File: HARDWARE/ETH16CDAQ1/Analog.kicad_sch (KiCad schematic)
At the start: 15 parts, among them J401 5499141-4, U401 ADG5408BRUZ, U402 ADG5408BRUZ, U403 ADA4254ARUZ

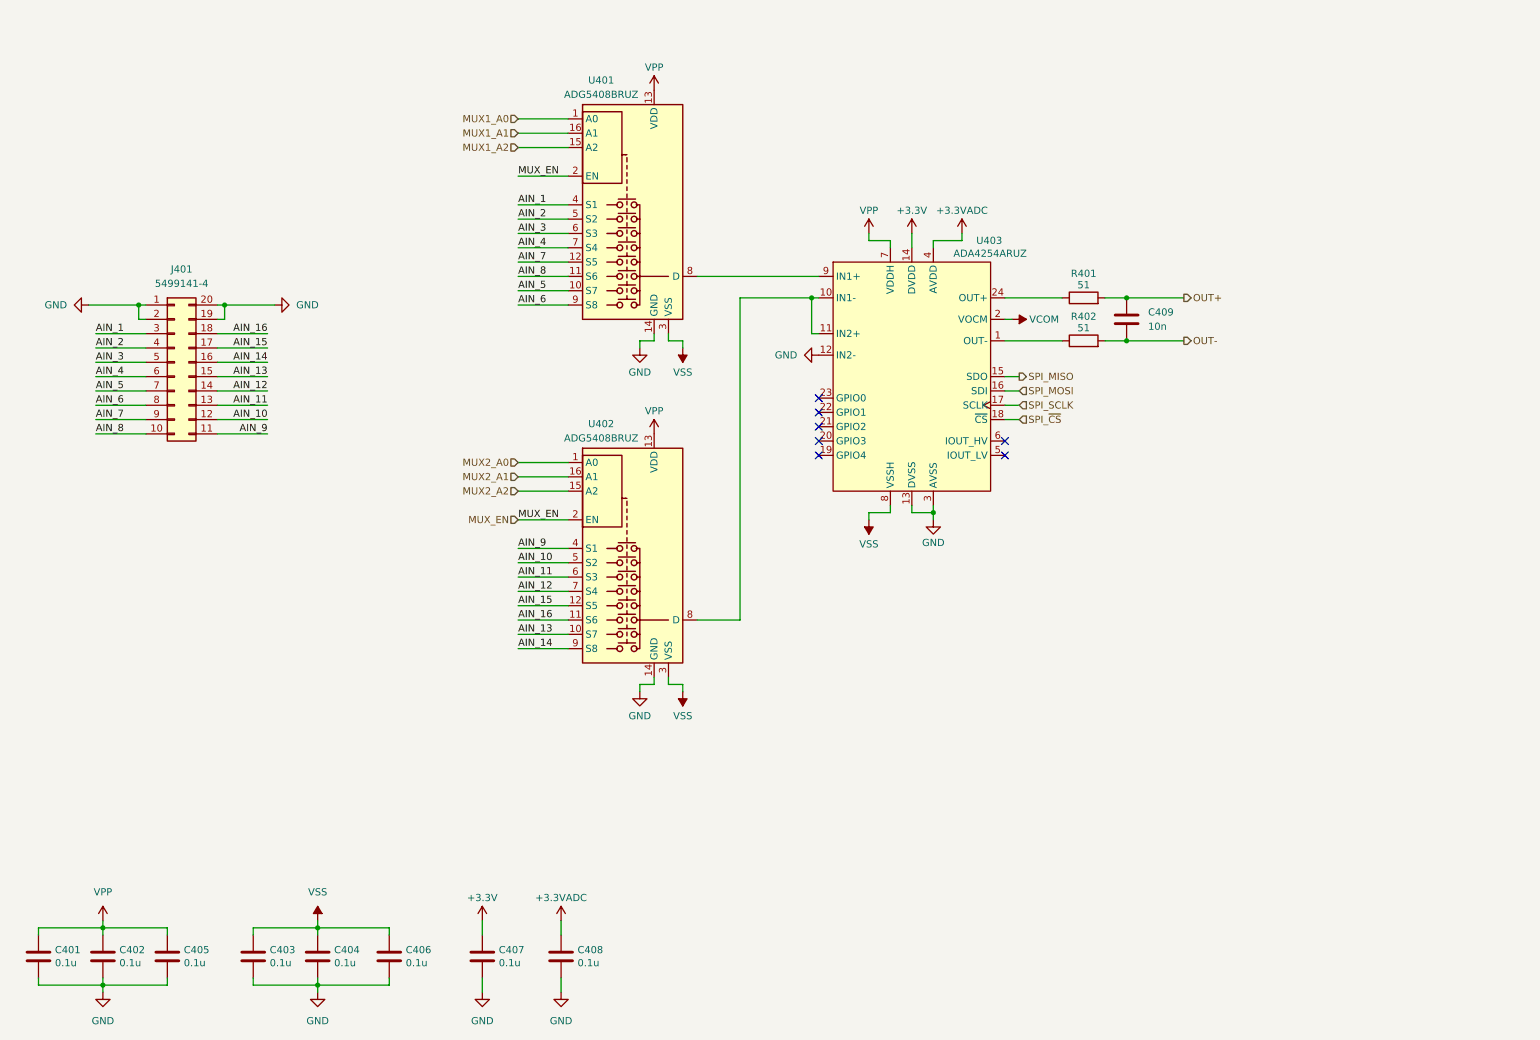
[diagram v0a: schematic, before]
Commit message: Development
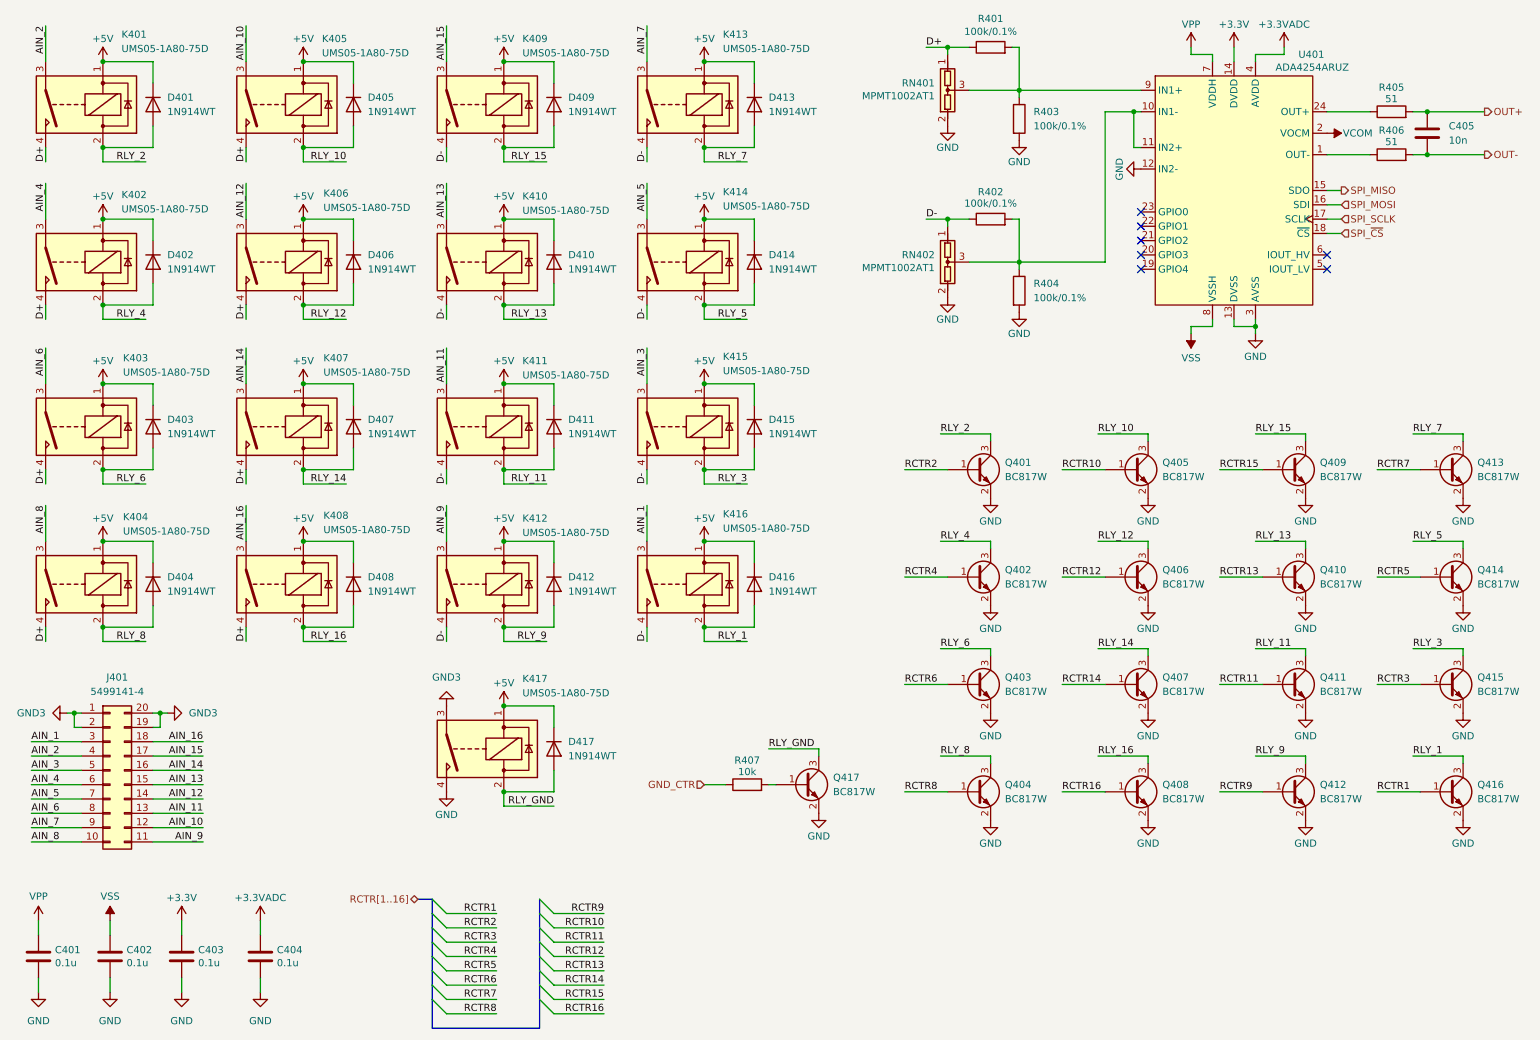
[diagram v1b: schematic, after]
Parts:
- removed C401, C403, C405, C406: 0.1u, Capacitor_SMD:C_0603_1608Metric_Pad1.08x0.95mm_HandSolder, symbol Device:C
- removed U401, U402: ADG5408BRUZ, Package_SO:TSSOP-16_4.4x5mm_P0.65mm, symbol Analog_Switch:ADG1408YRUZ
- added D401, D402, D403, D404, D405, D406, D407, D408, D409, D410, D411, D412, D413, D414, D415, D416, D417: 1N914WT, Diode_SMD:D_SOD-523, symbol Diode:1N914WT
- added K401, K402, K403, K404, K405, K406, K407, K408, K409, K410, K411, K412, K413, K414, K415, K416, K417: UMS05-1A80-75D, Relay_THT:Relay_StandexMeder_UMS, symbol Relay:UMS05-1A80-75D
- added Q401, Q402, Q403, Q404, Q405, Q406, Q407, Q408, Q409, Q410, Q411, Q412, Q413, Q414, Q415, Q416, Q417: BC817W, Package_TO_SOT_SMD:SOT-323_SC-70, symbol Transistor_BJT:BC817W
- added R401, R402, R403, R404: 100k/0.1%, Resistor_SMD:R_0805_2012Metric_Pad1.20x1.40mm_HandSolder, symbol Device:R
- added R407: 10k, Resistor_SMD:R_0603_1608Metric_Pad0.98x0.95mm_HandSolder, symbol Device:R
- added RN401, RN402: MPMT1002AT1, Package_TO_SOT_SMD:SOT-23, symbol Device:VoltageDivider_CenterPin3
- renumbered C402 to C401, C404 to C402, C407 to C403, C408 to C404, C409 to C405, R401 to R405, R402 to R406, U403 to U401
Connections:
- net AIN_1: now also K416.3
- net AIN_10: now also K405.3
- net AIN_11: now also K411.3
- net AIN_12: now also K406.3
- net AIN_13: now also K410.3
- net AIN_14: now also K407.3
- net AIN_15: now also K409.3
- net AIN_16: now also K408.3
- net AIN_2: now also K401.3
- net AIN_3: now also K415.3
- net AIN_4: now also K402.3
- net AIN_5: now also K414.3
- net AIN_6: now also K403.3
- net AIN_7: now also K413.3
- net AIN_8: now also K404.3
- net AIN_9: now also K412.3
- net GND: now also K417.4, Q401.2 (E), Q402.2 (E), Q403.2 (E), Q404.2 (E), Q405.2 (E), Q406.2 (E), Q407.2 (E), Q408.2 (E), Q409.2 (E), Q410.2 (E), Q411.2 (E), Q412.2 (E), Q413.2 (E), Q414.2 (E), Q415.2 (E), Q416.2 (E), Q417.2 (E), R403.2, R404.2, RN401.2, RN402.2; no longer J401.1 (Pin_1), J401.19 (Pin_19), J401.2 (Pin_2), J401.20 (Pin_20)
- net at U401.9 (IN1+): now also R401.2, R403.1, RN401.3
- net at U401.10 (IN1-), U401.11 (IN2+): now also R402.2, R404.1, RN402.3
- new net: Q417.1 (B), R407.2
- new net +5V: D401.1 (K), D402.1 (K), D403.1 (K), D404.1 (K), D405.1 (K), D406.1 (K), D407.1 (K), D408.1 (K), D409.1 (K), D410.1 (K), D411.1 (K), D412.1 (K), D413.1 (K), D414.1 (K), D415.1 (K), D416.1 (K), D417.1 (K), K401.1, K402.1, K403.1, K404.1, K405.1, K406.1, K407.1, K408.1, K409.1, K410.1, K411.1, K412.1, K413.1, K414.1, K415.1, K416.1, K417.1
- new net D+: K401.4, K402.4, K403.4, K404.4, K405.4, K406.4, K407.4, K408.4, R401.1, RN401.1
- new net D-: K409.4, K410.4, K411.4, K412.4, K413.4, K414.4, K415.4, K416.4, R402.1, RN402.1
- new net GND3: J401.1 (Pin_1), J401.19 (Pin_19), J401.2 (Pin_2), J401.20 (Pin_20), K417.3
- new net GND_CTR: R407.1
- new net RCTR1: Q416.1 (B)
- new net RCTR10: Q405.1 (B)
- new net RCTR11: Q411.1 (B)
- new net RCTR12: Q406.1 (B)
- new net RCTR13: Q410.1 (B)
- new net RCTR14: Q407.1 (B)
- new net RCTR15: Q409.1 (B)
- new net RCTR16: Q408.1 (B)
- new net RCTR2: Q401.1 (B)
- new net RCTR3: Q415.1 (B)
- new net RCTR4: Q402.1 (B)
- new net RCTR5: Q414.1 (B)
- new net RCTR6: Q403.1 (B)
- new net RCTR7: Q413.1 (B)
- new net RCTR8: Q404.1 (B)
- new net RCTR9: Q412.1 (B)
- new net RLY_1: D416.2 (A), K416.2, Q416.3 (C)
- new net RLY_10: D405.2 (A), K405.2, Q405.3 (C)
- new net RLY_11: D411.2 (A), K411.2, Q411.3 (C)
- new net RLY_12: D406.2 (A), K406.2, Q406.3 (C)
- new net RLY_13: D410.2 (A), K410.2, Q410.3 (C)
- new net RLY_14: D407.2 (A), K407.2, Q407.3 (C)
- new net RLY_15: D409.2 (A), K409.2, Q409.3 (C)
- new net RLY_16: D408.2 (A), K408.2, Q408.3 (C)
- new net RLY_2: D401.2 (A), K401.2, Q401.3 (C)
- new net RLY_3: D415.2 (A), K415.2, Q415.3 (C)
- new net RLY_4: D402.2 (A), K402.2, Q402.3 (C)
- new net RLY_5: D414.2 (A), K414.2, Q414.3 (C)
- new net RLY_6: D403.2 (A), K403.2, Q403.3 (C)
- new net RLY_7: D413.2 (A), K413.2, Q413.3 (C)
- new net RLY_8: D404.2 (A), K404.2, Q404.3 (C)
- new net RLY_9: D412.2 (A), K412.2, Q412.3 (C)
- new net RLY_GND: D417.2 (A), K417.2, Q417.3 (C)
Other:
- moved on the sheet: C401, C402, C403, C404, C405, J401, R405, R406, U401
